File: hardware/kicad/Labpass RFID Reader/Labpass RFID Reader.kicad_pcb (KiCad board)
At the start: 2 copper layers, 74 x 74 mm, 64 parts, among them J1 Conn_01x03_Male, J2 Conn_01x08, J3 Conn_01x02, J4 Conn_01x02, U1 adafruit_huzzah_32, U2 LM393, U3 LM324, U4 MFRC522, Y1 27.12 MHz

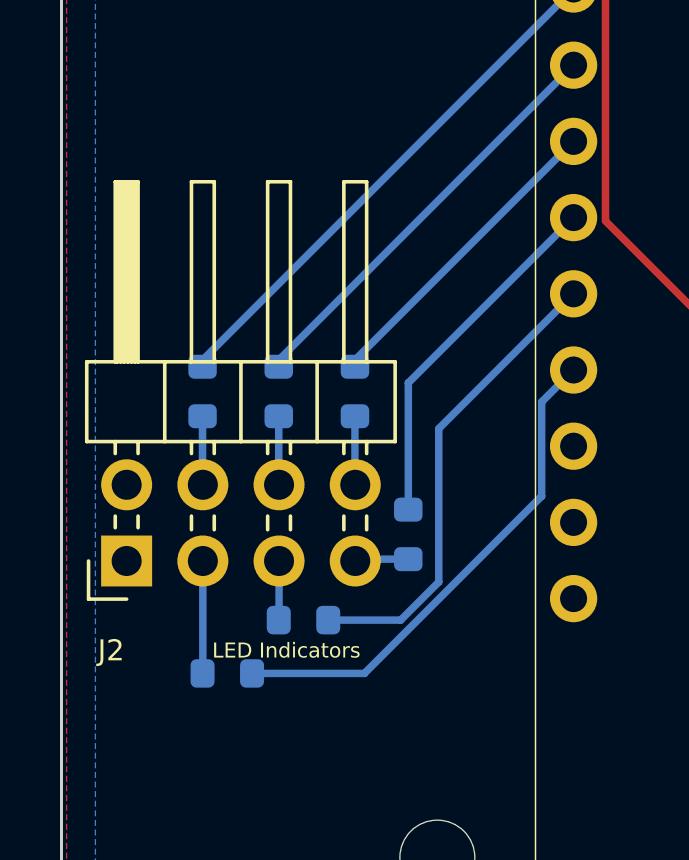
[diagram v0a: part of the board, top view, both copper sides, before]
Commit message: Final rev 1.0.0
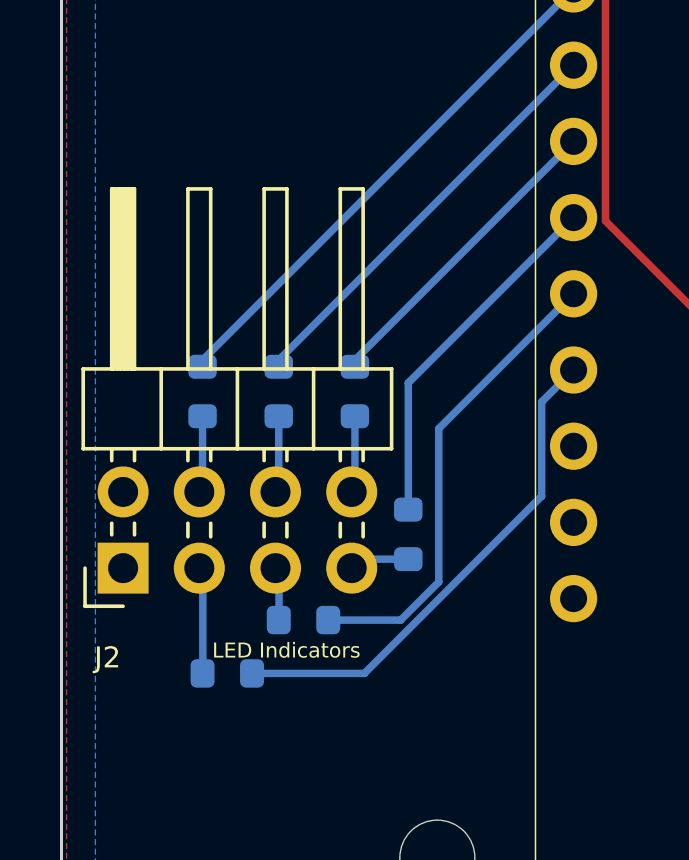
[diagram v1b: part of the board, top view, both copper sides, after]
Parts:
- moved J2 0.27 mm to (108.3, 114.6)
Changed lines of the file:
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@@
   )
   (footprint "Connector_PinHeader_2.54mm:PinHeader_2x04_P2.54mm_Horizontal" (layer "F.Cu")
-    (at 108.468 114.362 90)
+    (at 108.35 114.6 90)
     (descr "Through hole angled pin header, 2x04, 2.54mm pitch, 6mm pin length, double rows")
     (tags "Through hole angled pin header THT 2x04 2.54mm double row")
